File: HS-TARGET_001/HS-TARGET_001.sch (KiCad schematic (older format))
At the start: 43 parts, among them J1 5V_Serial, J2 i2c, J3 ICSP, J4 PROG, J5 dry_cell, Q1 Q_NMOS_GDS, Q2 Q_NMOS_GDS, Q3 Q_NMOS_GDS, SW1 RESET, SW2 SW_DIP_x04, U1 TSOP59540TR1, U2 ATmega328P-PU, U3 DFPLAYER_MINI, U4 TWELITE_DIP, U5 R-781.8-1.0, U6 AE-XCL102D503CR-G, Y1 Crystal

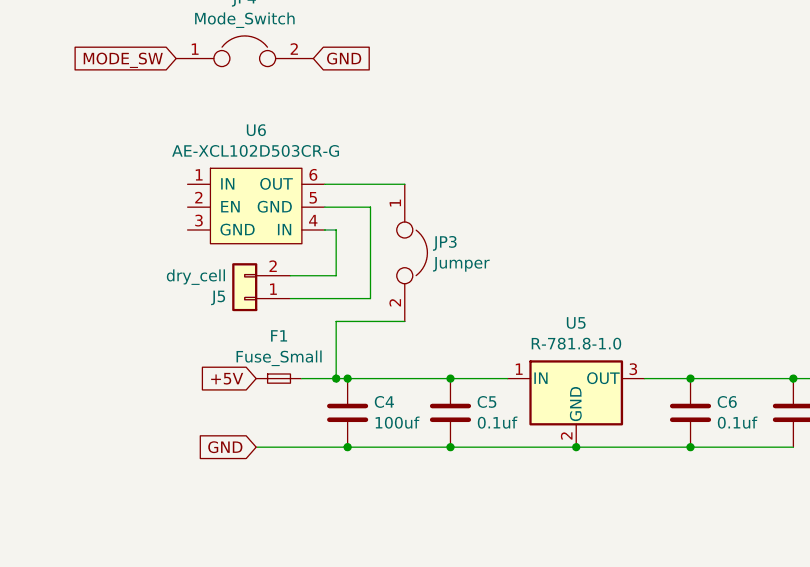
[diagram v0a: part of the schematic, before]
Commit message: ・HS-TARGET001基盤修正 ・HS-TAGLED001 開始
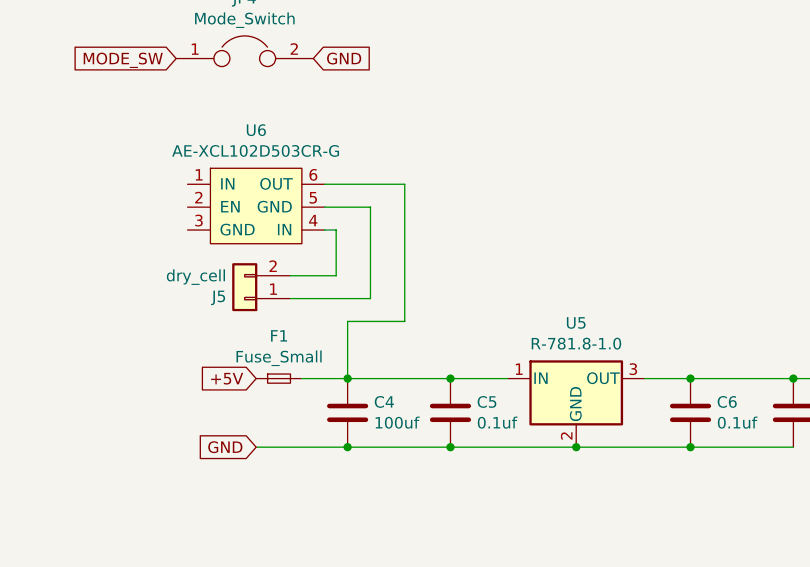
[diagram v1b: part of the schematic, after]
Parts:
- removed JP3: Jumper, Connector_PinHeader_2.54mm:PinHeader_1x02_P2.54mm_Vertical, symbol Device:Jumper
- SW1: footprint Button_Switch_THT:SW_TH_Tactile_Omron_B3F-10xx -> digikey-footprints:Switch_Tactile_THT_6x6mm
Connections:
- net at C4.1, C5.1, F1.2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: now also U6.6 (OUT)
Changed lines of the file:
@@
 F 0 "SW1" H 3800 3385 50  0000 C CNN
 F 1 "RESET" H 3800 3294 50  0000 C CNN
-F 2 "Button_Switch_THT:SW_TH_Tactile_Omron_B3F-10xx" H 3800 3150 50  0001 C CNN
+F 2 "digikey-footprints:Switch_Tactile_THT_6x6mm" H 3800 3150 50  0001 C CNN
 F 3 "~" H 3800 3150 50  0001 C CNN
 	1    3800 3150
@@
 $EndComp
 Connection ~ 7950 5750
-Wire Wire Line
-	7750 5750 7900 5750
 $Comp
 L HotSprings:AE-XCL102D503CR-G U6
@@
 	1    0    0    -1
 $EndComp
-$Comp
-L Device:Jumper JP3
-U 1 1 5D7BA38C
-P 8200 5200
-F 0 "JP3" V 8154 5327 50  0000 L CNN
-F 1 "Jumper" V 8245 5327 50  0000 L CNN
-F 2 "Connector_PinHeader_2.54mm:PinHeader_1x02_P2.54mm_Vertical" H 8200 5200 50  0001 C CNN
-F 3 "~" H 8200 5200 50  0001 C CNN
-	1    8200 5200
-	0    1    1    0
-$EndComp
 Wire Wire Line
 	7850 4900 8200 4900
-Wire Wire Line
-	8200 5500 7900 5500
-Wire Wire Line
-	7900 5500 7900 5750
-Connection ~ 7900 5750
-Wire Wire Line
-	7900 5750 7950 5750
 $Comp
 L Connector_Generic:Conn_01x02 J5
@@
 	7850 5000 8050 5000
 Wire Wire Line
-	8050 5000 8050 5400
-Wire Wire Line
-	8050 5400 7700 5400
-Wire Wire Line
 	7850 5100 7900 5100
-Wire Wire Line
-	7900 5100 7900 5300
-Wire Wire Line
-	7900 5300 7700 5300
 $Comp
 L Device:Jumper JP4
@@
 Text GLabel 7800 4350 2    50   Input ~ 0
 GND
+Wire Wire Line
+	8200 4900 8200 5500
+Wire Wire Line
+	7900 5300 7700 5300
+Wire Wire Line
+	7900 5100 7900 5300
+Wire Wire Line
+	8050 5400 7700 5400
+Wire Wire Line
+	8050 5000 8050 5400
+Wire Wire Line
+	7750 5750 7950 5750
+Wire Wire Line
+	8200 5500 7950 5500
+Wire Wire Line
+	7950 5500 7950 5750
 $EndSCHEMATC
